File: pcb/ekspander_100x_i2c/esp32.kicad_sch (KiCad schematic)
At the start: 11 parts, among them IC1 ESP32-S3-WROOM-1U-N16R8, U13 AP63203WU

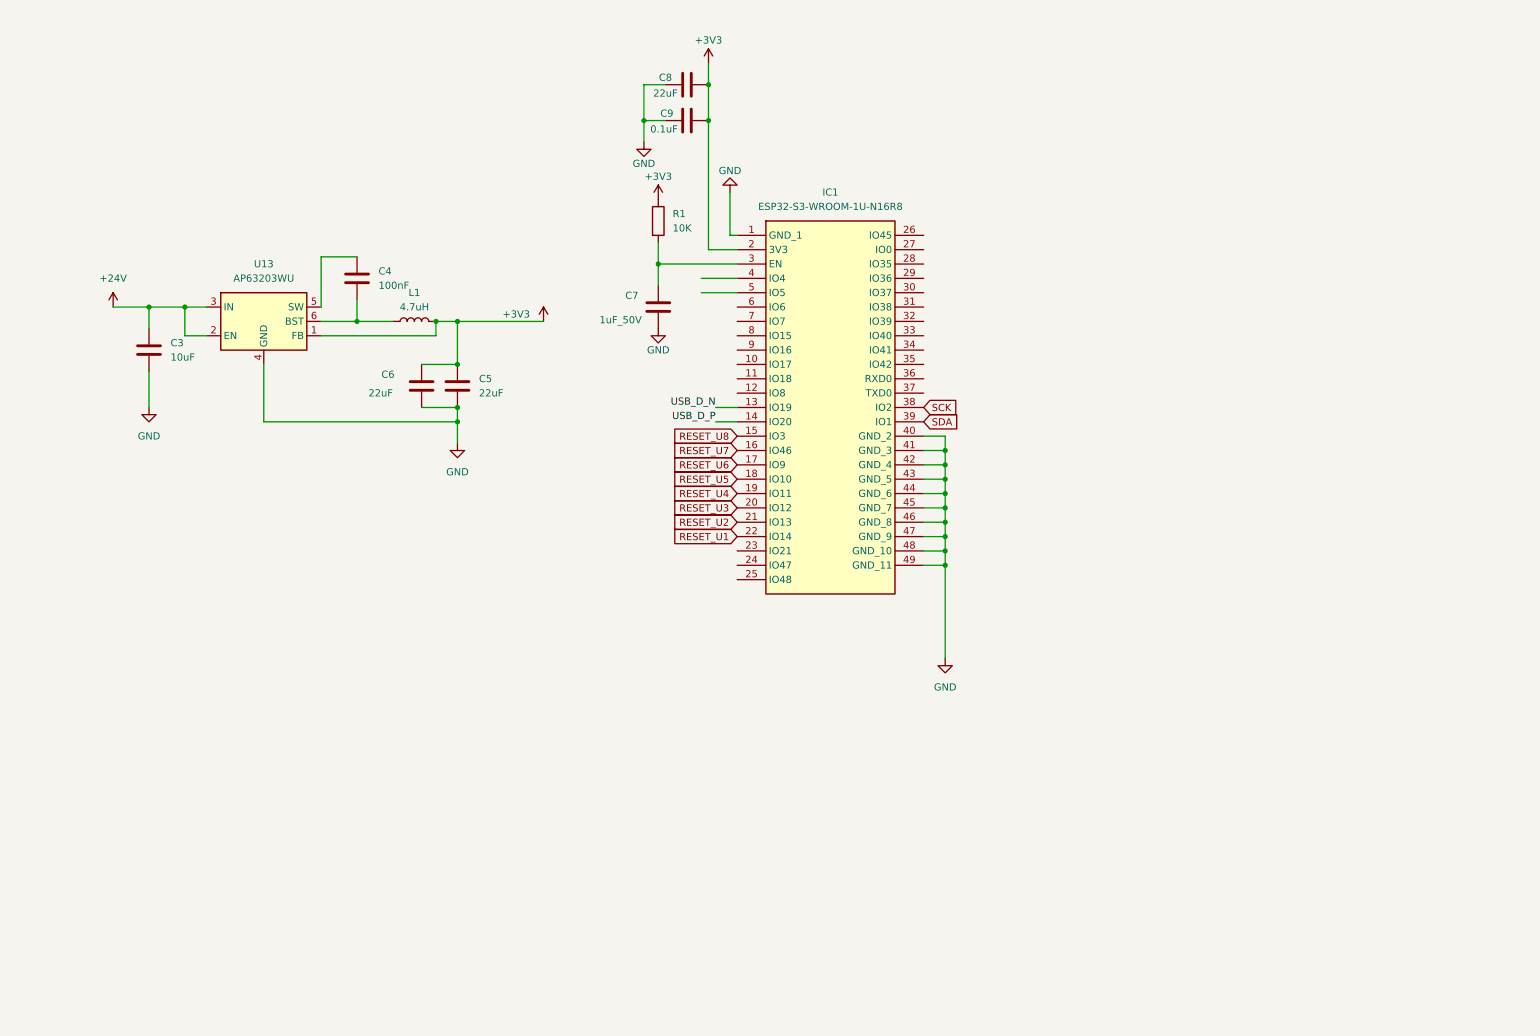
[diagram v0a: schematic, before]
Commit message: Ekspander 100x - UART-USB
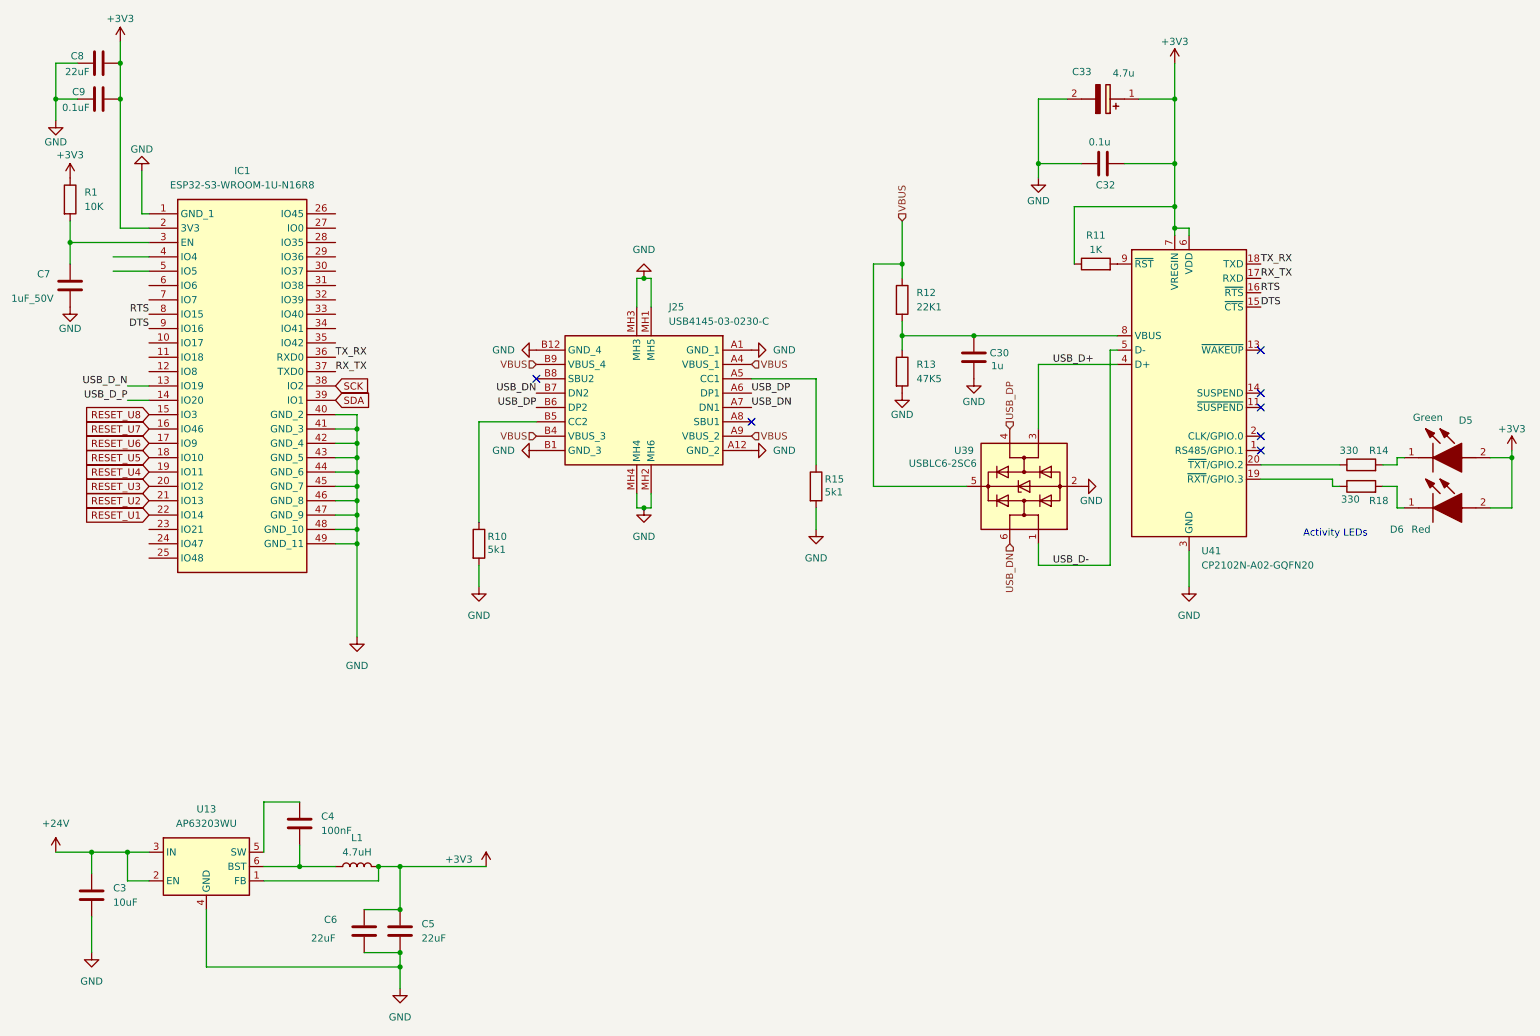
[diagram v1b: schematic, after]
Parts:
- added C30: 1u, Capacitor_SMD:C_0805_2012Metric, symbol SparkFun-Capacitor:C
- added C32: 0.1u, Capacitor_SMD:C_0805_2012Metric, symbol SparkFun-Capacitor:C
- added C33: 4.7u, Footprints:T491A, symbol T491A106K010AT7280:T491A106K010AT7280
- added D5: Green, 1_tme:LEDC2012X120N, symbol LTST-C170GKT:LTST-C170GKT
- added D6: Red, 1_tme:LEDC2012X120N, symbol LTST-C170KRKT:LTST-C170KRKT
- added J25: USB4145-03-0230-C, USB4145030230C, symbol 1_tme:USB4145-03-0230-C
- added R10, R15: 5k1, Resistor_SMD:R_0805_2012Metric, symbol Device:R
- added R11: 1K, Resistor_SMD:R_0805_2012Metric, symbol Device:R
- added R12: 22K1, Resistor_SMD:R_0805_2012Metric, symbol Device:R
- added R13: 47K5, Resistor_SMD:R_0805_2012Metric, symbol Device:R
- added R14, R18: 330, Resistor_SMD:R_0805_2012Metric, symbol Device:R
- added U39: USBLC6-2SC6, Package_TO_SOT_SMD:SOT-23-6, symbol Power_Protection:USBLC6-2SC6
- added U41: CP2102N-A02-GQFN20, Package_DFN_QFN:SiliconLabs_QFN-20-1EP_3x3mm_P0.5mm_EP1.8x1.8mm, symbol Interface_USB:CP2102N-Axx-xQFN20
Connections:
- net +3V3: now also C32.1, C33.1 (+), D5.2 (A), D6.2 (A), R11.1, U41.6 (VDD), U41.7 (VREGIN)
- net GND: now also C30.2, C32.2, C33.2 (-), J25.A1 (GND_1), J25.A12 (GND_2), J25.B1 (GND_3), J25.B12 (GND_4), J25.MH1 (MH5), J25.MH2 (MH6), J25.MH3, J25.MH4, R10.2, R13.2, R15.2, U39.2 (GND), U41.12 (GND), U41.21 (GND), U41.3 (GND)
- net TX_RX: now reaches IC1.36 (RXD0)
- net TX_RX: now also U41.18 (TXD)
- net RX_TX: now reaches IC1.37 (TXD0)
- net RX_TX: now also U41.17 (RXD)
- net RTS: now reaches IC1.8 (IO15)
- net RTS: now also U41.16 (~{RTS})
- net DTS: now reaches IC1.9 (IO16)
- net DTS: now also U41.15 (~{CTS})
- new net: J25.A5 (CC1), R15.1
- new net: C30.1, R12.2, R13.1, U41.8 (VBUS)
- new net: R18.1, U41.19 (~{RXT}/GPIO.3)
- new net: R14.1, U41.20 (~{TXT}/GPIO.2)
- new net: R11.2, U41.9 (~{RST})
- new net: J25.B5 (CC2), R10.1
- new net: D6.1 (K), R18.2
- new net: D5.1 (K), R14.2
- new net USB_D+: U39.3 (I/O2), U41.4 (D+)
- new net USB_D-: U39.1 (I/O1), U41.5 (D-)
- new net USB_DN: J25.A7 (DN1), J25.B7 (DN2), U39.6 (I/O1)
- new net USB_DP: J25.A6 (DP1), J25.B6 (DP2), U39.4 (I/O2)
- new net VBUS: J25.A4 (VBUS_1), J25.A9 (VBUS_2), J25.B4 (VBUS_3), J25.B9 (VBUS_4), R12.1, U39.5 (VBUS)
- no-connect marks 0 -> 7
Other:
- note added: "Activity LEDs"
- moved on the sheet: C3, C4, C5, C6, C7, C8, C9, IC1, L1, R1, U13
